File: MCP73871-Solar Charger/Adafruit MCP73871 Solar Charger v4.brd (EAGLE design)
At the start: 40.7 x 33 mm, 35 parts, among them CN1 DCIN, IC1 MCP73871

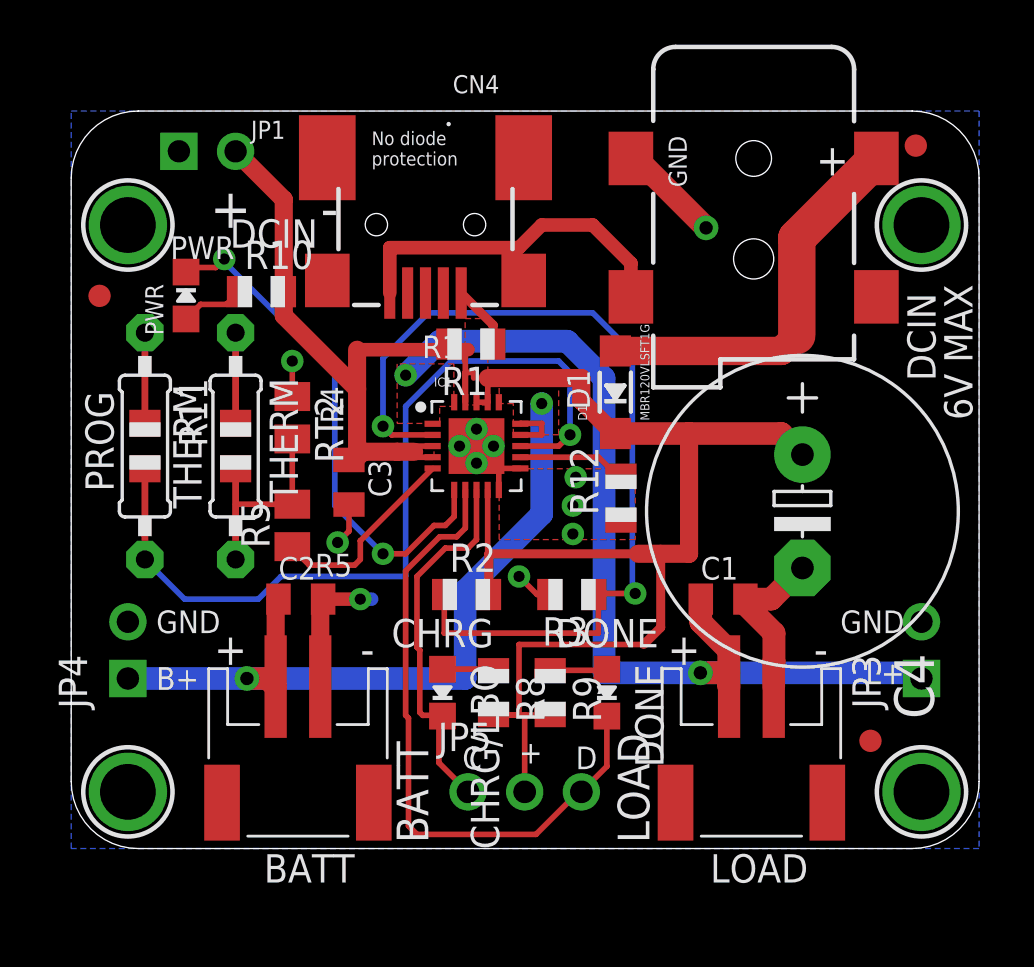
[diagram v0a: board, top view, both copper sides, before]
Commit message: Fix Silkscreen issues with Solar board
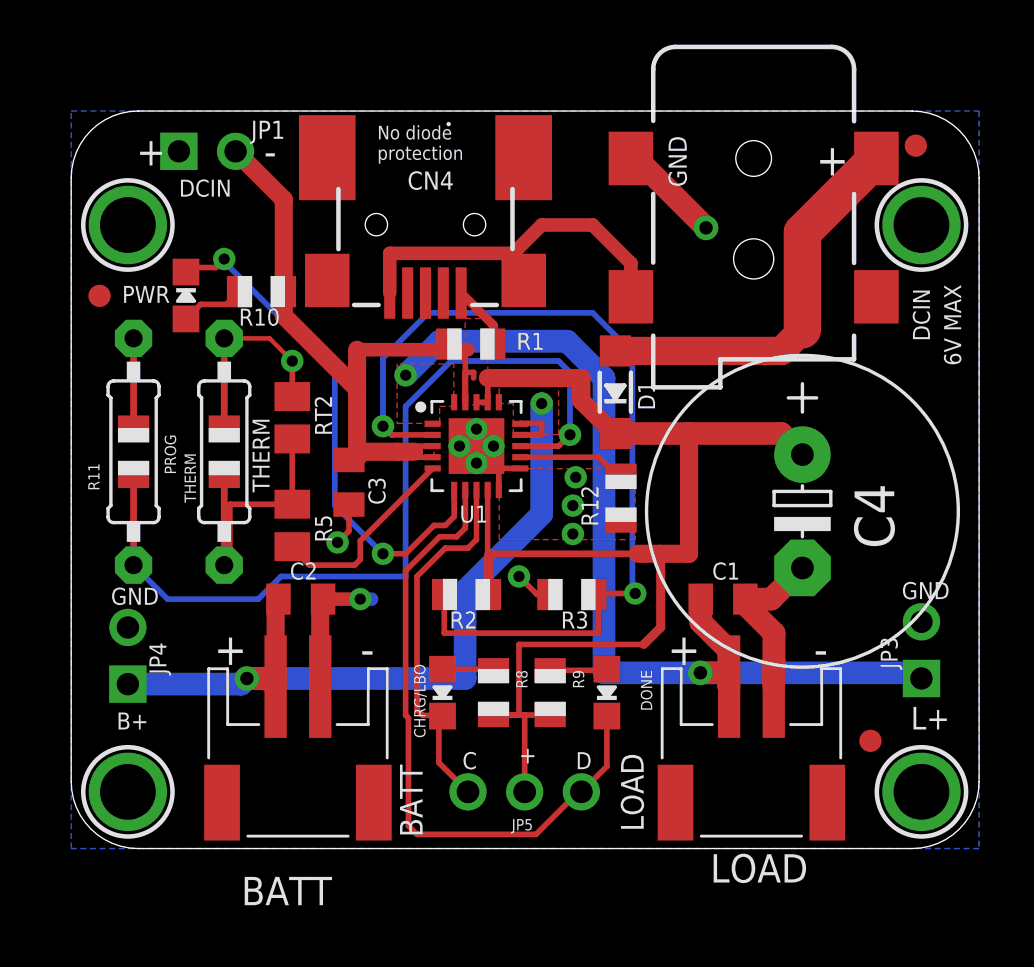
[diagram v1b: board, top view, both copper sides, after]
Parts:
- moved R11 0.57 mm to (2.79, 17.8)
- moved THERM 0.57 mm to (6.86, 17.8)
- moved JP4 0.25 mm to (2.54, 8.64)
- renumbered IC1 to U1
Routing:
- net GND: track 27.5 -> 31.0 mm
- net N$8: track 7.94 -> 8.55 mm
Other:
- board text removed: "D1"
- board text removed: "PWR"
- board text removed: "R1"
- board text removed: "R4"
- board text removed: "R5"
